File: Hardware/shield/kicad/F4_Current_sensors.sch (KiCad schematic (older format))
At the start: 26 parts, among them U3 MCP6244

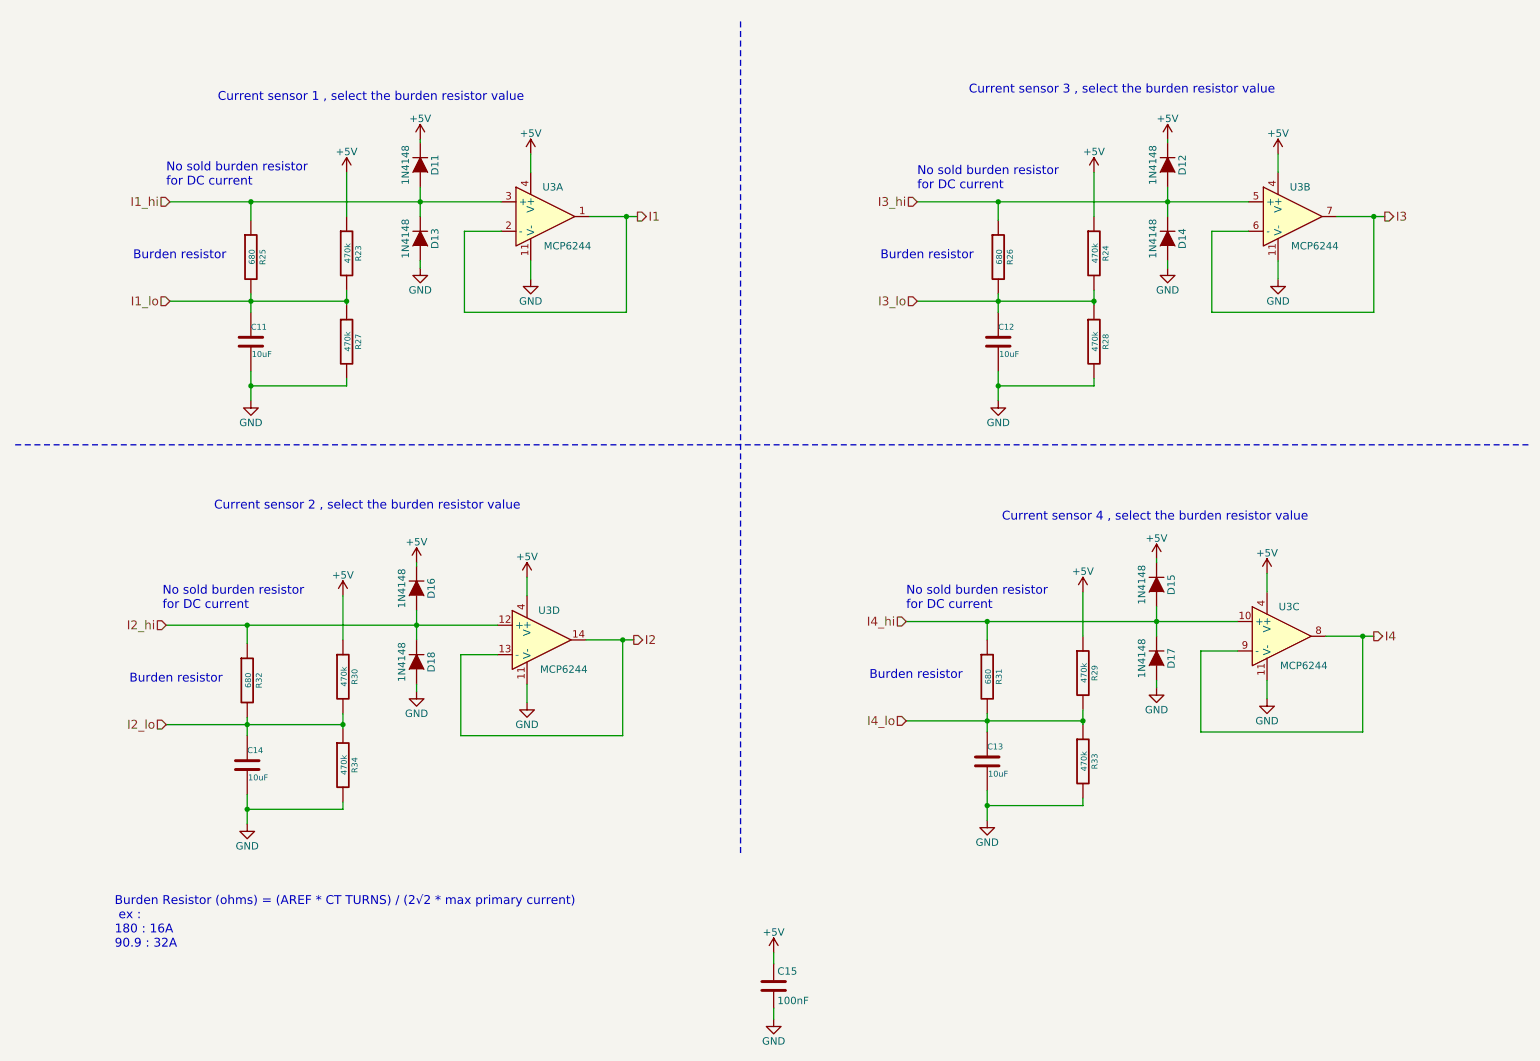
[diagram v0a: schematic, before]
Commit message: move to digital 1.1.1
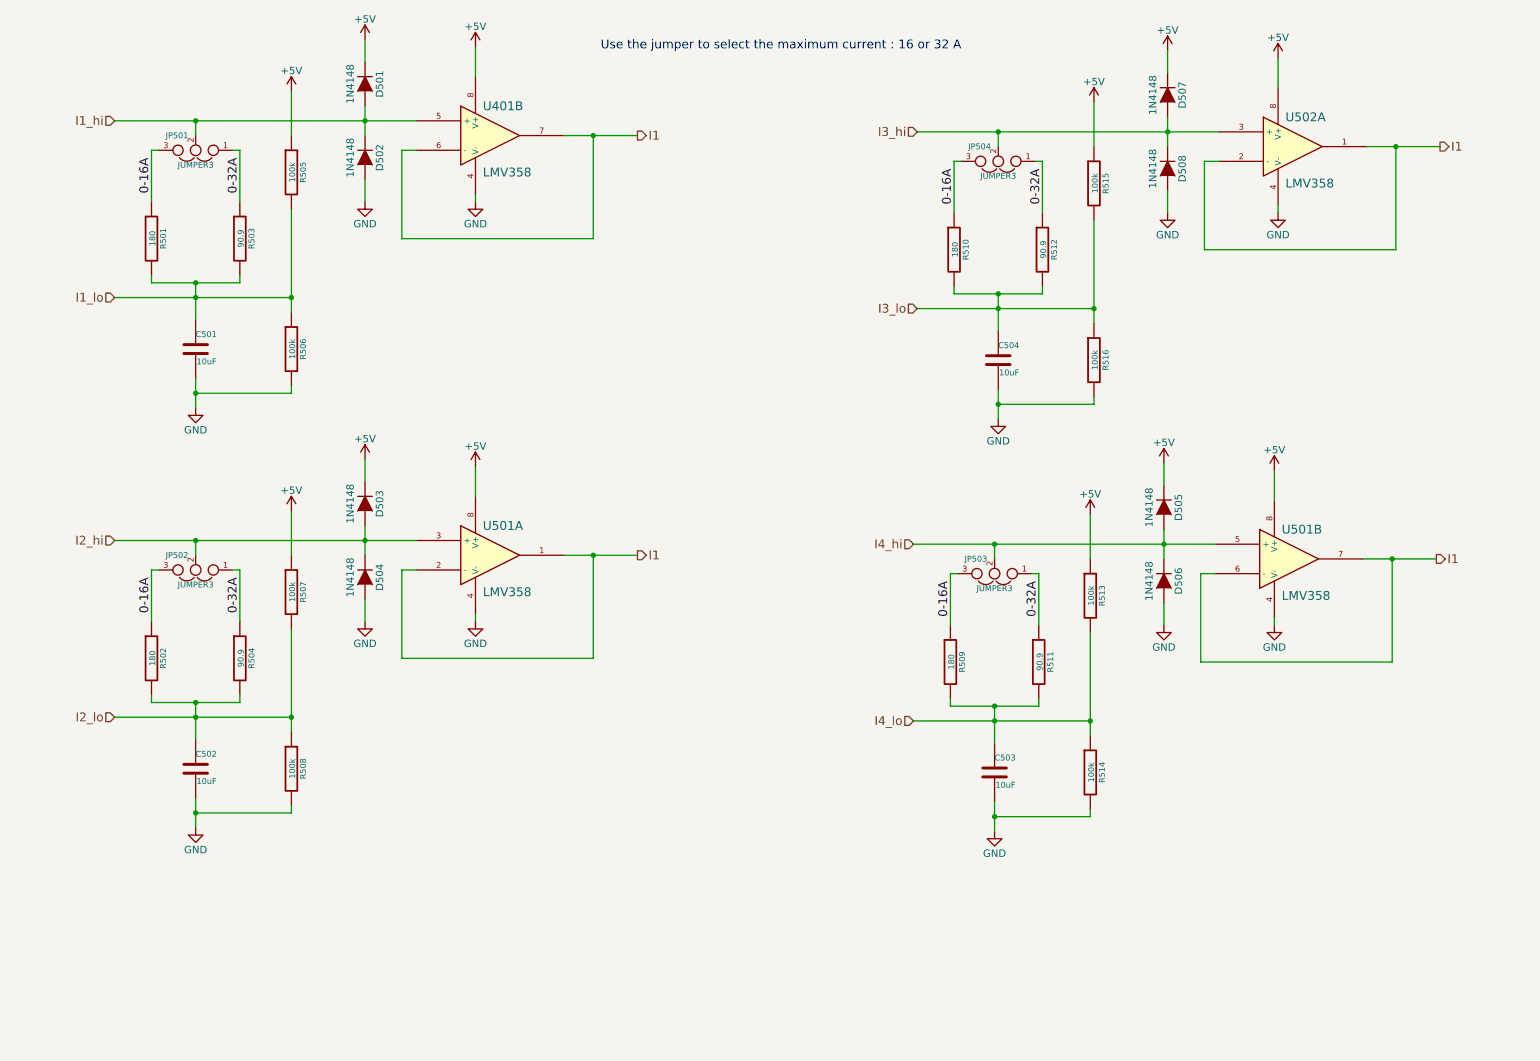
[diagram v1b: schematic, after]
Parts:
- removed C12, C13, C14: 10uF, Capacitors_ThroughHole:C_Radial_D5_L6_P2.5, symbol C-RESCUE-Windlogger
- removed C15: 100nF, Capacitors_ThroughHole:C_Rect_L7_W2.5_P5, symbol C
- removed D12, D14, D15, D16, D17, D18: 1N4148, Discret:DO-35, symbol D
- removed R24, R28, R29, R30, R33, R34: 470k, Discret:R3-LARGE_PADS, symbol R-RESCUE-Windlogger
- removed R26, R31, R32: 680, Discret:R3-LARGE_PADS, symbol R-RESCUE-Windlogger
- removed U3: MCP6244, Housings_DIP:DIP-14_W7.62mm_LongPads, symbol MCP6004
- added C502, C503, C504: 10uF, Capacitors_ThroughHole:C_Radial_D5_L6_P2.5, symbol C-RESCUE-Windlogger
- added D503, D504, D505, D506, D507, D508: 1N4148, Diodes_ThroughHole:Diode_DO-35_SOD27_Horizontal_RM10, symbol D
- added JP501, JP502, JP503, JP504: JUMPER3, Pin_Headers:Pin_Header_Straight_1x03, symbol JUMPER3
- added R502, R509, R510: 180, Discret:R4, symbol R-RESCUE-Windlogger
- added R503, R504, R511, R512: 90.9, Discret:R4, symbol R-RESCUE-Windlogger
- added R507, R508, R513, R514, R515, R516: 100k, Discret:R4, symbol R-RESCUE-Windlogger
- added U401, U501, U502: LMV358, Housings_DIP:DIP-8_W7.62mm_LongPads, symbol LM358-RESCUE-Windlogger
- D501: renamed from D11; footprint Discret:DO-35 -> Diodes_ThroughHole:Diode_DO-35_SOD27_Horizontal_RM10
- D502: renamed from D13; footprint Discret:DO-35 -> Diodes_ThroughHole:Diode_DO-35_SOD27_Horizontal_RM10
- R501: renamed from R25; value 680 -> 180; footprint Discret:R3-LARGE_PADS -> Discret:R4
- R505: renamed from R23; value 470k -> 100k; footprint Discret:R3-LARGE_PADS -> Discret:R4
- R506: renamed from R27; value 470k -> 100k; footprint Discret:R3-LARGE_PADS -> Discret:R4
- renumbered C11 to C501
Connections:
- net +5V: now also D503.1 (K), D505.1 (K), D507.1 (K), R507.1, R513.1, R515.1, U401.8 (V+), U501.8 (V+), U501.8 (V+), U502.8 (V+)
- net GND: now also C502.2, C503.2, C504.2, D504.2 (A), D506.2 (A), D508.2 (A), R508.2, R514.2, R516.2, U401.4 (V-), U501.4 (V-), U501.4 (V-), U502.4 (V-)
- net I1: now also U401.6 (-), U401.7, U501.1, U501.2 (-), U501.6 (-), U501.7, U502.1, U502.2 (-)
- net I1_hi: now also JP501.2, U401.5 (+); no longer R501.1
- net I1_lo: now also R503.2
- net I2_hi: now also D503.2 (A), D504.1 (K), JP502.2, U501.3 (+)
- net I2_lo: now also C502.1, R502.2, R504.2, R507.2, R508.1
- net I3_hi: now also D507.2 (A), D508.1 (K), JP504.2, U502.3 (+)
- net I3_lo: now also C504.1, R510.2, R512.2, R515.2, R516.1
- net I4_hi: now also D505.2 (A), D506.1 (K), JP503.2, U501.5 (+)
- net I4_lo: now also C503.1, R509.2, R511.2, R513.2, R514.1
- new net 0-16A: JP501.3, JP502.3, JP503.3, JP504.3, R501.1, R502.1, R509.1, R510.1
- new net 0-32A: JP501.1, JP502.1, JP503.1, JP504.1, R503.1, R504.1, R511.1, R512.1
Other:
- note added: "Use the jumper to select the maximum current : 16 or 32 A\n"
- note removed: "Burden Resistor (ohms) = (AREF * CT TURNS) / (2√2 * max primary current)\n ex :\n180 : 16A\n90.9 : 32A\n"
- note removed: "Burden resistor"
- note removed: "Current sensor 1 , select the burden resistor value"
- note removed: "Current sensor 2 , select the burden resistor value"
- note removed: "Current sensor 3 , select the burden resistor value"
- note removed: "Current sensor 4 , select the burden resistor value"
- note removed: "No sold burden resistor\nfor DC current"
- moved on the sheet: C501, D501, D502, R501, R505, R506
